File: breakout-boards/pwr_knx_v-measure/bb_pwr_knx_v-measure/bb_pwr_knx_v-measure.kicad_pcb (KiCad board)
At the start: 2 copper layers, 28.5 x 25 mm, 50 parts, among them IC1 TPS560430, T1 BC856, T2 FZT753, T3 BC847

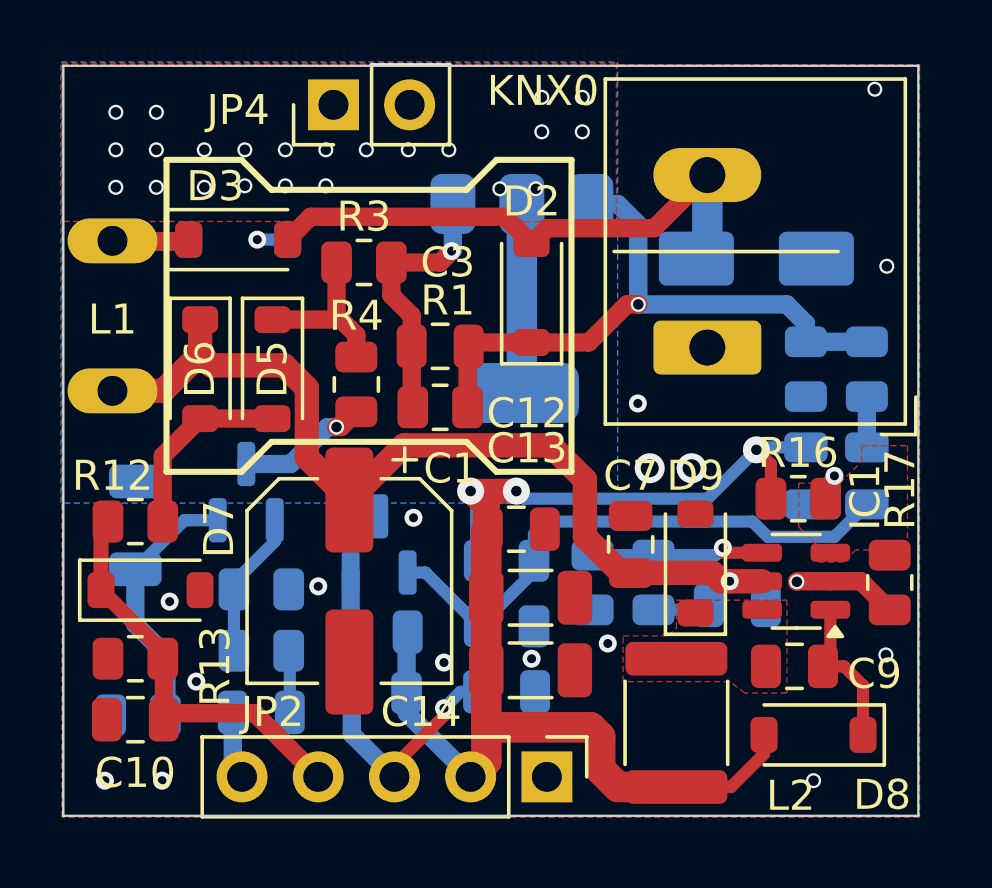
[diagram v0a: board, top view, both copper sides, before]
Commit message: finally standardize selected parts on all boards
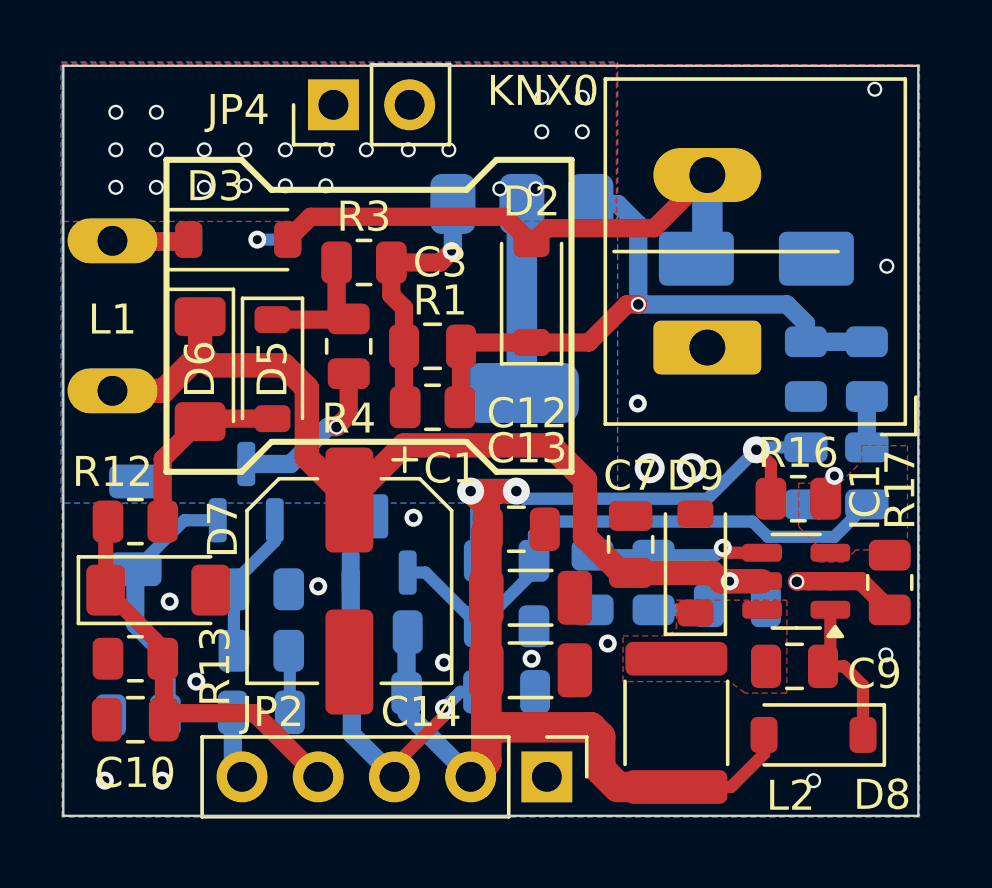
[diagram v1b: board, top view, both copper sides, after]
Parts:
- D6, D7: footprint Diode_SMD:D_SOD-123 -> Diode_SMD:D_MiniMELF
- R13: value 6,2k -> 6k2
- R25: value 24R 1W -> 24R 1W
- moved R4 1.30 mm to (143.8, 101.9)
- moved D7 0.26 mm to (137.4, 110.0)
- moved C3 0.25 mm to (146.6, 101.9)
- moved R1 0.25 mm to (146.6, 103.9)
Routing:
- net Net-(D5-K): track 5.71 -> 4.51 mm
- net Net-(T3-C): track 4.55 -> 5.50 mm
